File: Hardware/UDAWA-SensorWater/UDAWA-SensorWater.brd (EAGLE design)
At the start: 160 x 100 mm, 9 parts

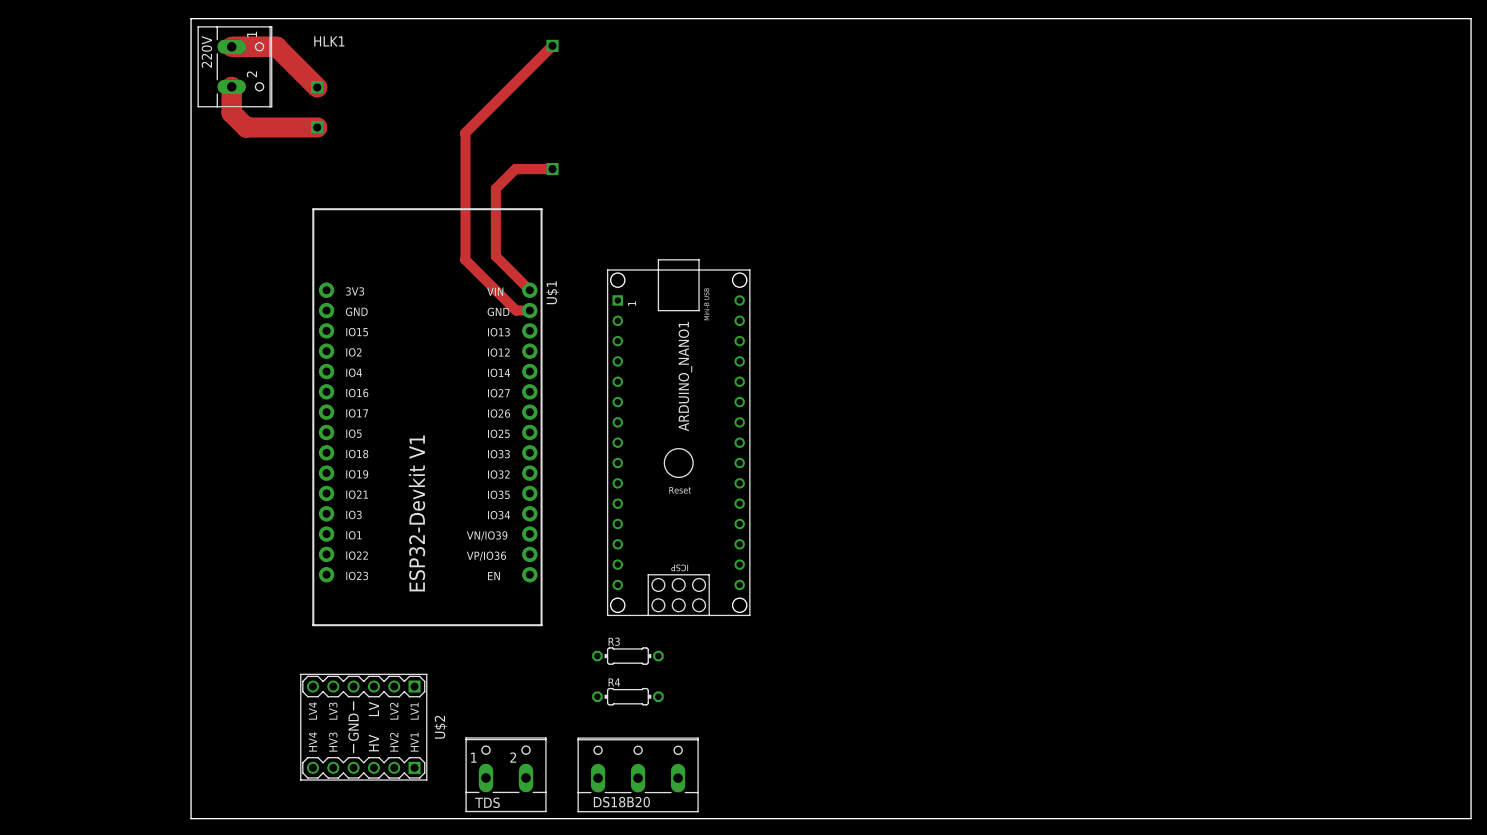
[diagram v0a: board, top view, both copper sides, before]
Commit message: First working version of Water Sensor
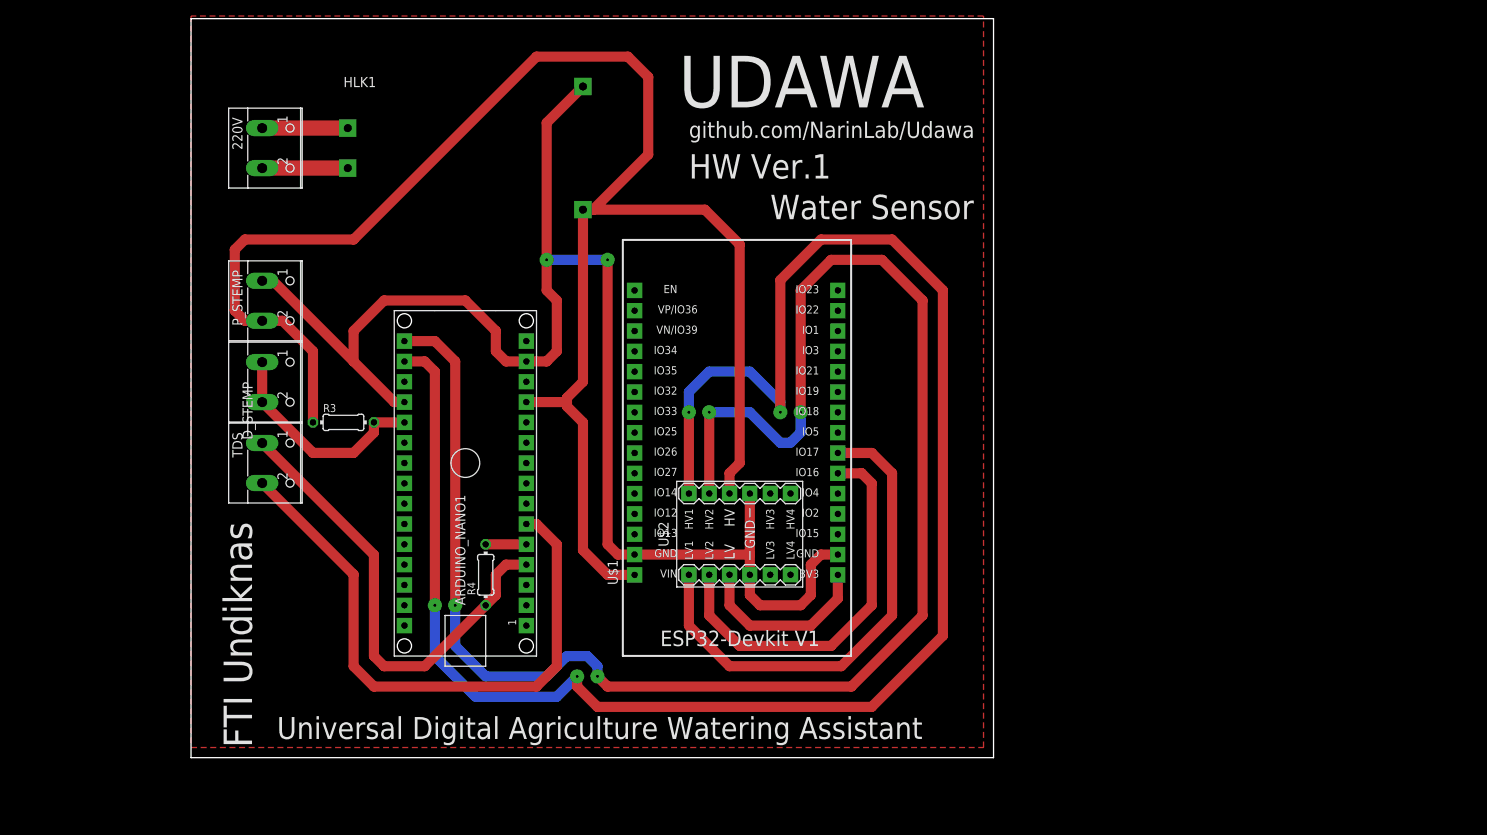
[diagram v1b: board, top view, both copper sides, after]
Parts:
- removed DS18B20: (no value), con-wago-500:W237-103
- added D_STEMP, P_STEMP: (no value), con-wago-500:W237-102
- moved U$2 52.8 mm to (68.6, 35.6), turned to 90 degrees
- moved TDS 48.0 mm to (10.2, 44.5), turned to 270 degrees
- moved R3 46.0 mm to (19.1, 49.5)
- moved U$1 39.5 mm to (68.6, 47.0), turned to 90 degrees
- moved ARDUINO_NANO1 26.7 mm to (34.3, 44.5), turned to 90 degrees
- moved R4 23.4 mm to (36.8, 30.5), turned to 90 degrees
- moved 220V 10.9 mm to (10.2, 83.8)
- moved HLK1 6.35 mm to (34.3, 83.8)
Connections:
- net 5V: now also P_STEMP.2; no longer DS18B20.3
- net D2: now also D_STEMP.1, D_STEMP.2; no longer DS18B20.2
- net GND: now also P_STEMP.1; no longer DS18B20.1
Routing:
- net HV1: track 0.00 -> 225.3 mm, vias 0 -> 4
- net HV2: track 0.00 -> 209.8 mm, vias 0 -> 4
- net 5V: track 22.5 -> 221.9 mm
- net GND: track 41.9 -> 186.1 mm, vias 0 -> 2
- net A2: track 0.00 -> 75.2 mm
- net LV1: track 0.00 -> 62.1 mm
- net A0: track 0.00 -> 58.7 mm
- net LV2: track 0.00 -> 49.1 mm
- net D2: track 0.00 -> 27.7 mm
- net 3V3: track 0.00 -> 22.8 mm
- net A1: track 0.00 -> 5.08 mm
- net AC2: track 14.7 -> 10.7 mm
- net AC1: track 12.8 -> 10.7 mm
- added copper zone on layer 1, net GND
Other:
- board size 160 x 100 mm -> 100.3 x 92.4 mm
- board text added: "FTI Undiknas"
- board text added: "HW Ver.1"
- board text added: "UDAWA"
- board text added: "Universal Digital Agriculture Watering Assistant"
- board text added: "Water Sensor"
- board text added: "github.com/NarinLab/Udawa"
